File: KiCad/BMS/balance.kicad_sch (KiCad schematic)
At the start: 121 parts, among them Q1 PNP, Q10 NMOS, Q11 PNP, Q12 BSS138, Q13 NMOS, Q14 PNP, Q15 NMOS, Q16 PNP, Q17 NMOS, Q2 NMOS, Q3 PNP, Q4 NMOS, Q5 PNP, Q6 NMOS, Q7 PNP, Q8 NMOS, Q9 PNP, U10 TL431A, U11 B0505MT, U12 MCP3201, U13 TL431A, U14 HCPL-0630, U15 TL431A, U16 HCPL-0600, U17 TL431A, U18 HCPL-0600, U19 TL431A, U20 TL431A, U5 TL431A, U6 HCPL-0630, U7 74HC4051, U8 TL431A, U9 HCPL-0630

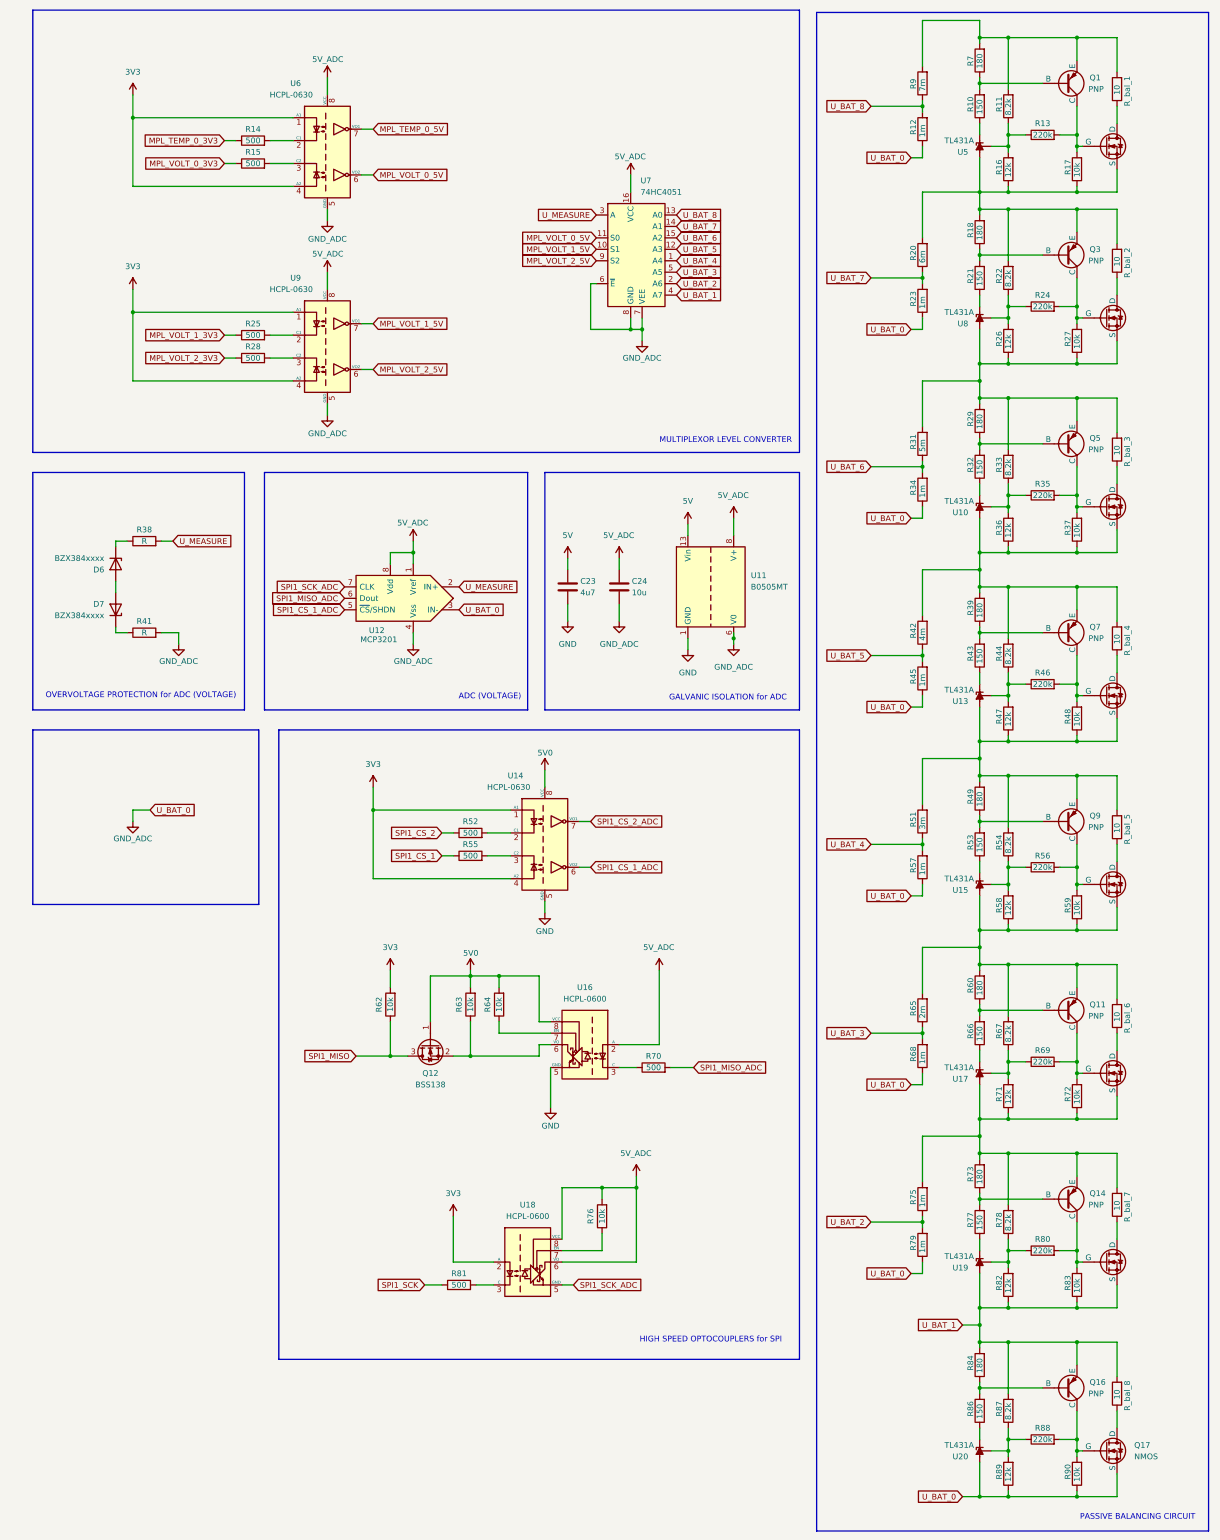
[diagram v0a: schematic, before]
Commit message: 22.03.2025
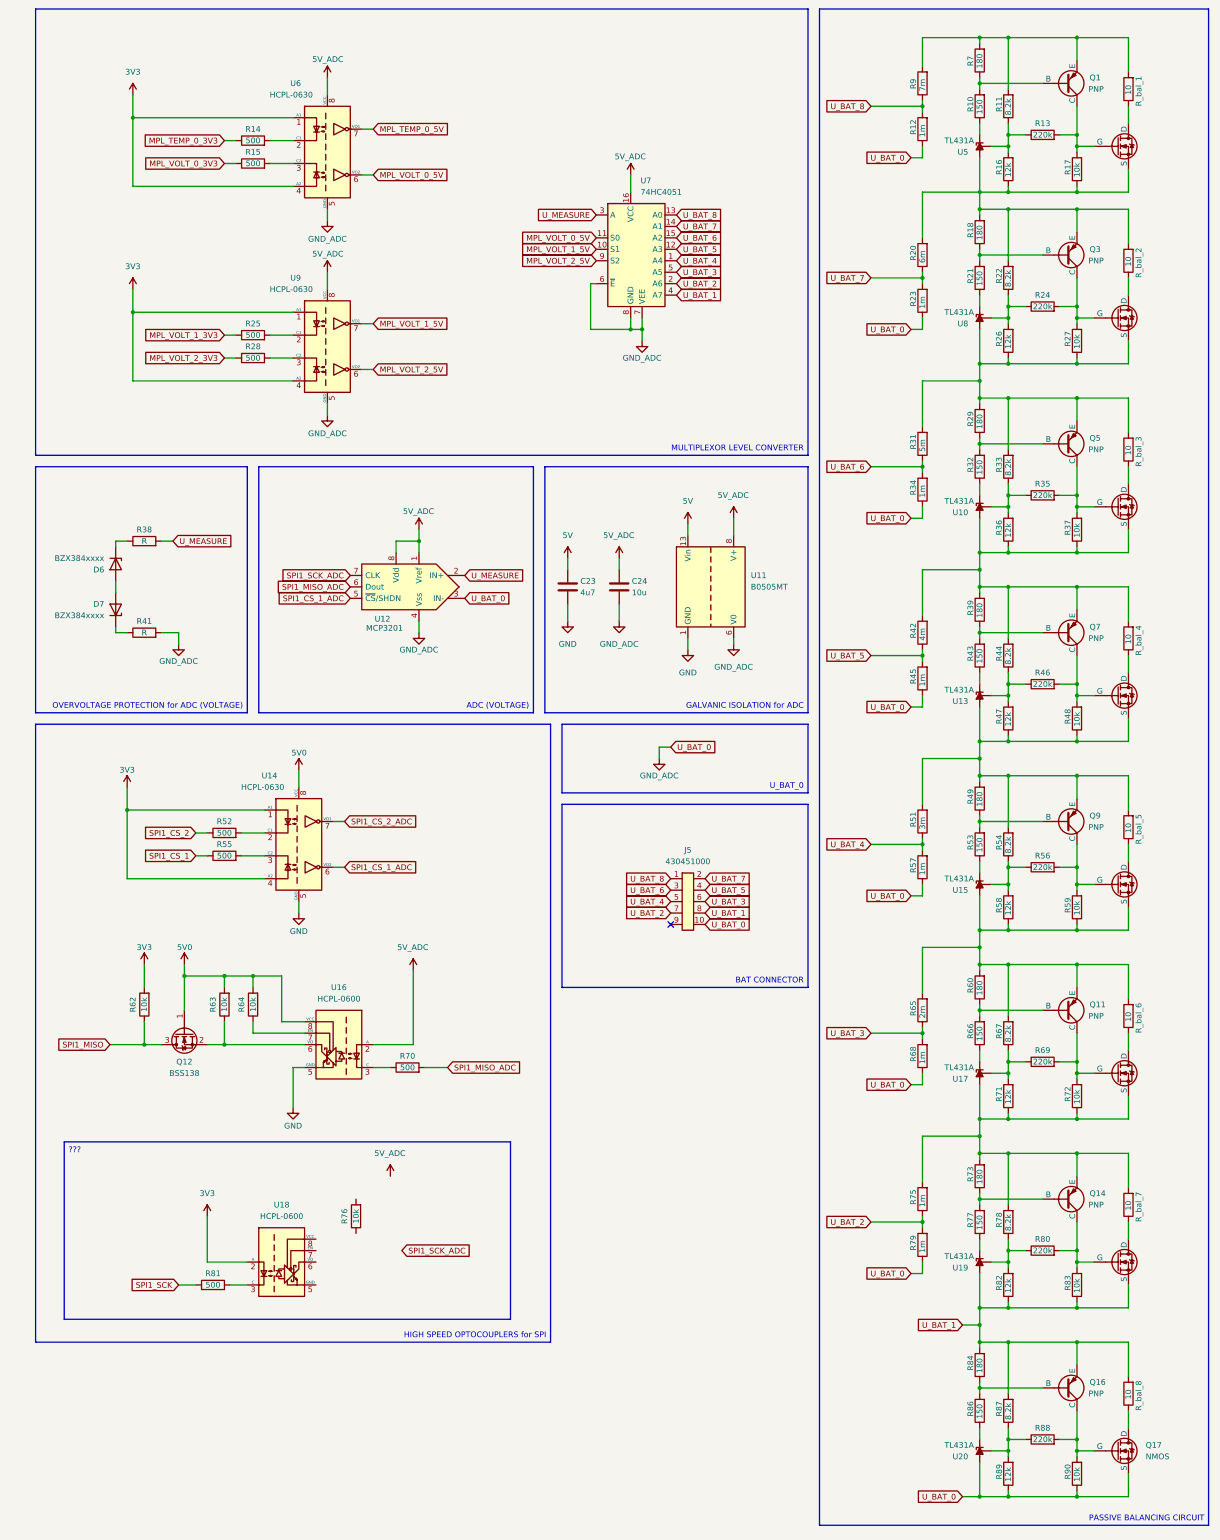
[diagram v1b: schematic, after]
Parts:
- added J5: 430451000, Connector_Molex:Molex_Micro-Fit_3.0_43045-1000_2x05_P3.00mm_Horizontal, symbol user_lib:430451200
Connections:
- net 5V_ADC: no longer R76.2, U18.6 (VO), U18.8 (VCC)
- net GND_ADC: now also J5.10
- net SPI1_SCK_ADC: no longer U18.5 (GND)
- net U_BAT_1: now also J5.8
- net U_BAT_2: now also J5.7
- net U_BAT_3: now also J5.6
- net U_BAT_4: now also J5.5
- net U_BAT_5: now also J5.4
- net U_BAT_6: now also J5.3
- net U_BAT_7: now also J5.2
- net U_BAT_8: now also J5.1
- net at R76.1: no longer U18.7 (EN)
- no-connect marks 0 -> 1
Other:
- note removed: "ADC (VOLTAGE)"
- note removed: "GALVANIC ISOLATION for ADC"
- note removed: "HIGH SPEED OPTOCOUPLERS for SPI"
- note removed: "MULTIPLEXOR LEVEL CONVERTER"
- note removed: "OVERVOLTAGE PROTECTION for ADC (VOLTAGE)"
- note removed: "PASSIVE BALANCING CIRCUIT"
- moved on the sheet: Q12, Q17, R52, R55, R62, R63, R64, R70, R76, R81, R_bal_1, R_bal_2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
